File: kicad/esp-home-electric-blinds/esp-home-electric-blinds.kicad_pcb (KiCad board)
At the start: 2 copper layers, 66.1 x 91 mm, 14 parts, among them J1 AC_IN, J2 Stepper_2_conn, J3 Stepper_2_conn, J4 Conn_01x05, U1 ESP32_mini, U2 TMC2208_Stepper_driver, U3 TMC2208_Stepper_driver

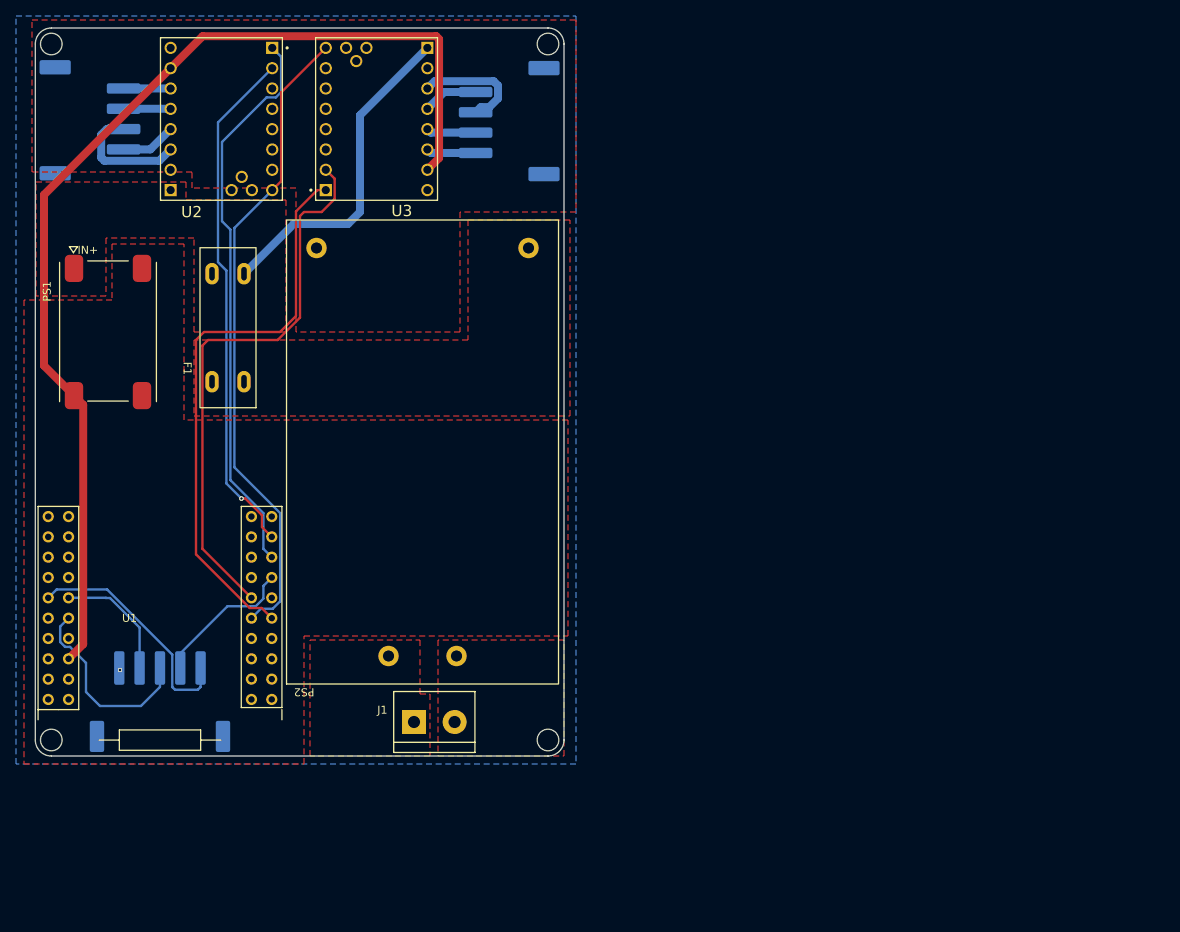
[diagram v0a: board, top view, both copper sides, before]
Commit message: pcb V2
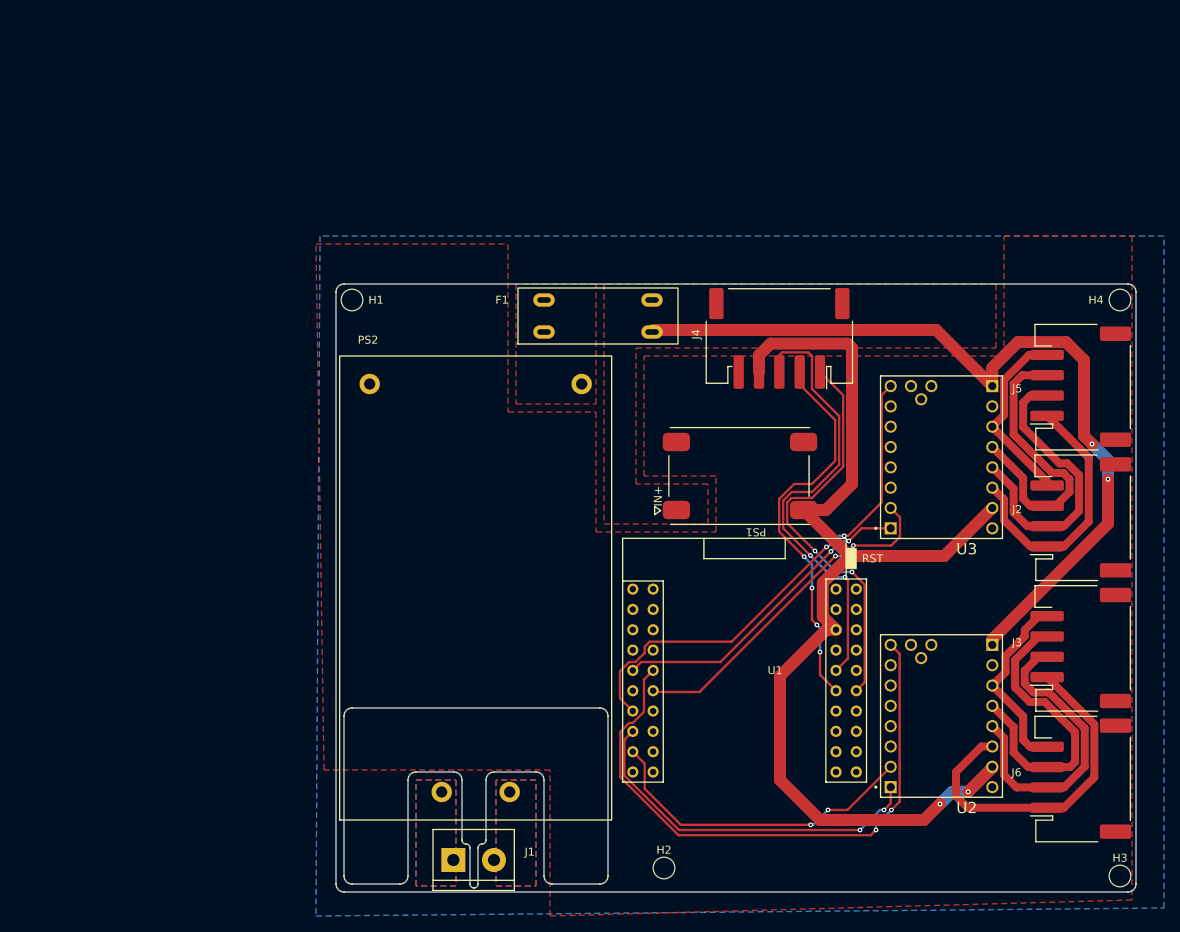
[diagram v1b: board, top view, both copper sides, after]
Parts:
- added J5: Stepper_2_conn, connectors_johnymalina:JST_smd_1x04_horizontal, F.Cu at (193.1, 86.7)
- added J6: Stepper_1_conn, connectors_johnymalina:JST_smd_1x04_horizontal, F.Cu at (193.1, 135.7)
- J2, J4: moved to F.Cu
- J3: value Stepper_2_conn -> Stepper_1_conn; moved to F.Cu
- moved H4 144.5 mm to (198.0, 76.0)
- moved J3 140.4 mm to (193.1, 119.3)
- moved U2 116.9 mm to (175.7, 128.0), turned to 180 degrees
- moved H2 104.0 mm to (141.0, 147.0)
- moved J4 89.8 mm to (155.4, 80.8)
- moved J2 86.7 mm to (193.1, 103.0), turned to 90 degrees
- moved U3 82.3 mm to (175.7, 95.7)
- moved PS1 81.0 mm to (150.5, 98.0), turned to 90 degrees
- moved U1 73.6 mm to (151.1, 123.6), turned to 180 degrees
- moved H3 73.5 mm to (198.0, 148.0)
- moved H1 49.4 mm to (102.0, 76.0)
- moved F1 46.3 mm to (132.8, 78.0), turned to 90 degrees
- moved PS2 18.3 mm to (117.5, 112.0)
- moved J1 17.9 mm to (114.7, 146.0)
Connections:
- J4 pad 2: IO_32 -> IO_19
- J4 pad 4: IO_19 -> +3.3V
- U1 pad 28: IO_32 -> EN_PIN_2
- U2 pad JP2_3: Net-(J3-Pin_2) -> Net-(J3-Pin_4)
- U2 pad JP2_4: Net-(J3-Pin_1) -> Net-(J3-Pin_3)
- U2 pad JP2_5: Net-(J3-Pin_3) -> Net-(J3-Pin_2)
- U2 pad JP2_6: Net-(J3-Pin_4) -> Net-(J3-Pin_1)
- U3 pad JP1_8: EN_PIN -> EN_PIN_2
- U3 pad JP2_3: Net-(J2-Pin_2) -> Net-(J2-Pin_4)
- U3 pad JP2_4: Net-(J2-Pin_1) -> Net-(J2-Pin_3)
- U3 pad JP2_5: Net-(J2-Pin_3) -> Net-(J2-Pin_2)
- U3 pad JP2_6: Net-(J2-Pin_4) -> Net-(J2-Pin_1)
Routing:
- net +12V: track 41.7 -> 104.4 mm, vias 0 -> 2
- net EN_PIN_2: track 0.00 -> 62.6 mm, vias 0 -> 2
- net Net-(J3-Pin_1): track 6.93 -> 43.3 mm
- net IO_19: track 15.7 -> 48.8 mm, vias 0 -> 4
- net IO_23: track 24.4 -> 56.5 mm, vias 0 -> 2
- net Net-(J3-Pin_3): track 5.88 -> 37.8 mm
- net DIR_PIN_2: track 71.2 -> 39.6 mm, vias 0 -> 2
- net Net-(J2-Pin_3): track 6.21 -> 36.8 mm
- net STEP_PIN_2: track 69.7 -> 43.0 mm, vias 0 -> 2
- net Net-(J2-Pin_1): track 6.90 -> 33.3 mm
- net DIR_PIN: track 70.4 -> 45.5 mm, vias 0 -> 2
- net STEP_PIN: track 64.5 -> 40.9 mm, vias 1 -> 2
- net Net-(J3-Pin_2): track 15.4 -> 38.2 mm
- net Net-(J2-Pin_2): track 14.6 -> 36.8 mm
- net IO_33: track 29.3 -> 51.1 mm, vias 0 -> 2
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- added copper zone on B.Cu, net AC_L
- added copper zone on B.Cu, net AC_N
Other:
- board size 66.1 x 91 mm -> 100 x 76 mm
- board text removed: "ESPHome Electric Blinds Author:Jakub Cihanek 26.03.2024 V2.0"
